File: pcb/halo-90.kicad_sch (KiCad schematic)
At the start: 102 parts, among them J1 TC2030-SWIM-NL, U1 UFQFPN28, U3 DRV5032

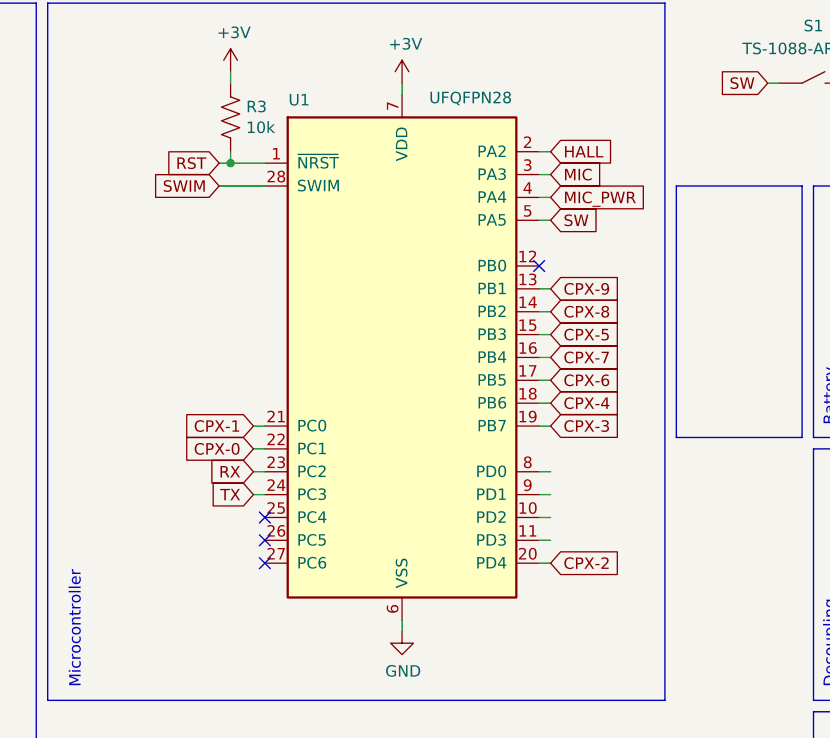
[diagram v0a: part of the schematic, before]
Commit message: WIP: Current hardware updates
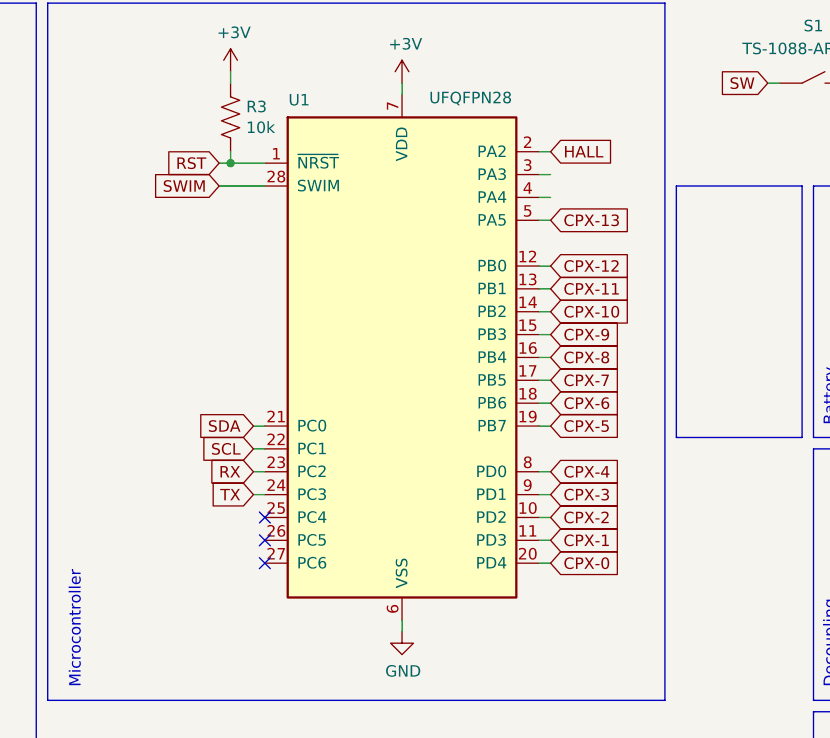
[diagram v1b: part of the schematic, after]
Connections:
- net CPX-0: now also U1.20 (PD4); no longer U1.22 (PC1)
- net CPX-1: now also U1.11 (PD3); no longer U1.21 (PC0)
- net CPX-2: now also U1.10 (PD2); no longer U1.20 (PD4)
- net CPX-3: now also U1.9 (PD1); no longer U1.19 (PB7)
- net CPX-4: now also U1.8 (PD0); no longer U1.18 (PB6)
- net CPX-5: now also U1.19 (PB7); no longer U1.15 (PB3)
- net CPX-6: now also U1.18 (PB6); no longer U1.17 (PB5)
- net CPX-7: now also U1.17 (PB5); no longer U1.16 (PB4)
- net CPX-8: now also U1.16 (PB4); no longer U1.14 (PB2)
- net CPX-9: now also U1.15 (PB3); no longer U1.13 (PB1)
- net MIC: no longer U1.3 (PA3)
- net MIC_PWR: no longer U1.4 (PA4)
- net SW: no longer U1.5 (PA5)
- net CPX-12: now reaches U1.12 (PB0)
- new net CPX-10: U1.14 (PB2)
- new net CPX-11: U1.13 (PB1)
- new net CPX-13: U1.5 (PA5)
- new net SCL: U1.22 (PC1)
- new net SDA: U1.21 (PC0)
- no-connect marks 24 -> 23
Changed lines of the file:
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@@
 	)
 	(no_connect
-		(at 228.6 43.18)
-	)
-	(no_connect
 		(at 198.12 71.12)
 	)
@@
 		)
 	)
+	(wire
+		(pts
+			(xy 228.6 43.18) (xy 229.87 43.18)
+		)
+		(stroke
+			(width 0)
+			(type default)
+		)
+	)
 	(polyline
 		(pts
@@
 	(global_label "CPX-5"
 		(shape input)
-		(at 229.87 50.8 0)
+		(at 229.87 60.96 0)
 		(effects
 			(font
@@
 		)
 		(property "Intersheetrefs" "${INTERSHEET_REFS}"
-			(at 162.56 -34.29 0)
+			(at 162.56 -24.13 0)
 			(effects
 				(font
@@
 	(global_label "CPX-3"
 		(shape input)
-		(at 229.87 60.96 0)
+		(at 229.87 68.58 0)
 		(effects
 			(font
@@
 		)
 		(property "Intersheetrefs" "${INTERSHEET_REFS}"
-			(at 162.56 8.89 0)
+			(at 162.56 16.51 0)
 			(effects
 				(font
@@
 		)
 	)
+	(global_label "CPX-11"
+		(shape input)
+		(at 229.87 45.72 0)
+		(effects
+			(font
+				(size 1.27 1.27)
+			)
+			(justify left)
+		)
+		(property "Intersheetrefs" "${INTERSHEET_REFS}"
+			(at 162.56 -29.21 0)
+			(effects
+				(font
+					(size 1.27 1.27)
+				)
+				(hide yes)
+			)
+		)
+	)
 	(global_label "CPX-9"
 		(shape input)
@@
 		)
 	)
-	(global_label "CPX-0"
+	(global_label "CPX-13"
 		(shape input)
-		(at 196.85 63.5 180)
+		(at 229.87 38.1 0)
 		(effects
 			(font
 				(size 1.27 1.27)
 			)
-			(justify right)
+			(justify left)
 		)
 		(property "Intersheetrefs" "${INTERSHEET_REFS}"
-			(at 264.16 107.95 0)
+			(at 162.56 -31.75 0)
 			(effects
 				(font
@@
 		)
 	)
-	(global_label "SW"
+	(global_label "CPX-0"
 		(shape input)
-		(at 229.87 38.1 0)
+		(at 229.87 76.2 0)
 		(effects
 			(font
@@
 		)
 		(property "Intersheetrefs" "${INTERSHEET_REFS}"
-			(at 162.56 -41.91 0)
+			(at 162.56 120.65 0)
 			(effects
 				(font
@@
 		)
 	)
-	(global_label "CPX-8"
+	(global_label "CPX-10"
 		(shape input)
 		(at 229.87 48.26 0)
@@
 		)
 		(property "Intersheetrefs" "${INTERSHEET_REFS}"
-			(at 162.56 -26.67 0)
+			(at 162.56 1.27 0)
+			(effects
+				(font
+					(size 1.27 1.27)
+				)
+				(hide yes)
+			)
+		)
+	)
+	(global_label "CPX-8"
+		(shape input)
+		(at 229.87 53.34 0)
+		(effects
+			(font
+				(size 1.27 1.27)
+			)
+			(justify left)
+		)
+		(property "Intersheetrefs" "${INTERSHEET_REFS}"
+			(at 162.56 -21.59 0)
 			(effects
 				(font
@@
 	(global_label "CPX-4"
 		(shape input)
-		(at 229.87 58.42 0)
+		(at 229.87 66.04 0)
 		(effects
 			(font
@@
 		)
 		(property "Intersheetrefs" "${INTERSHEET_REFS}"
-			(at 162.56 -24.13 0)
+			(at 162.56 -16.51 0)
 			(effects
 				(font
@@
 		)
 	)
-	(global_label "MIC"
+	(global_label "SDA"
 		(shape input)
-		(at 229.87 33.02 0)
+		(at 196.85 60.96 180)
 		(effects
 			(font
 				(size 1.27 1.27)
 			)
-			(justify left)
+			(justify right)
 		)
 		(property "Intersheetrefs" "${INTERSHEET_REFS}"
-			(at 162.56 -46.99 0)
+			(at 264.16 -19.05 0)
 			(effects
 				(font
@@
 	(global_label "CPX-9"
 		(shape input)
-		(at 229.87 45.72 0)
+		(at 229.87 50.8 0)
 		(effects
 			(font
@@
 		)
 		(property "Intersheetrefs" "${INTERSHEET_REFS}"
-			(at 162.56 -24.13 0)
+			(at 162.56 -19.05 0)
 			(effects
 				(font
@@
 		)
 	)
-	(global_label "MIC_PWR"
+	(global_label "SCL"
 		(shape input)
-		(at 229.87 35.56 0)
+		(at 196.85 63.5 180)
 		(effects
 			(font
 				(size 1.27 1.27)
 			)
-			(justify left)
+			(justify right)
 		)
 		(property "Intersheetrefs" "${INTERSHEET_REFS}"
-			(at 162.56 -44.45 0)
+			(at 264.16 -16.51 0)
 			(effects
 				(font
@@
 	(global_label "CPX-6"
 		(shape input)
-		(at 229.87 55.88 0)
+		(at 229.87 58.42 0)
 		(effects
 			(font
@@
 		)
 		(property "Intersheetrefs" "${INTERSHEET_REFS}"
-			(at 162.56 -31.75 0)
+			(at 162.56 -29.21 0)
 			(effects
 				(font
@@
 	(global_label "CPX-7"
 		(shape input)
-		(at 229.87 53.34 0)
+		(at 229.87 55.88 0)
 		(effects
 			(font
@@
 		)
 		(property "Intersheetrefs" "${INTERSHEET_REFS}"
-			(at 162.56 6.35 0)
+			(at 162.56 8.89 0)
 			(effects
 				(font
@@
 		)
 	)
+	(global_label "CPX-12"
+		(shape input)
+		(at 229.87 43.18 0)
+		(effects
+			(font
+				(size 1.27 1.27)
+			)
+			(justify left)
+		)
+		(property "Intersheetrefs" "${INTERSHEET_REFS}"
+			(at 162.56 -26.67 0)
+			(effects
+				(font
+					(size 1.27 1.27)
+				)
+				(hide yes)
+			)
+		)
+	)
 	(global_label "MIC"
 		(shape input)
@@
 	(global_label "CPX-1"
 		(shape input)
-		(at 196.85 60.96 180)
+		(at 229.87 73.66 0)
 		(effects
 			(font
 				(size 1.27 1.27)
 			)
-			(justify right)
+			(justify left)
 		)
 		(property "Intersheetrefs" "${INTERSHEET_REFS}"
-			(at 264.16 110.49 0)
+			(at 162.56 123.19 0)
 			(effects
 				(font
@@
 	(global_label "CPX-2"
 		(shape input)
-		(at 229.87 76.2 0)
+		(at 229.87 71.12 0)
 		(effects
 			(font
@@
 		)
 		(property "Intersheetrefs" "${INTERSHEET_REFS}"
-			(at 162.56 11.43 0)
+			(at 162.56 6.35 0)
 			(effects
 				(font
